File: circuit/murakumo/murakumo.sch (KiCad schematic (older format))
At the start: 105 parts, among them J1 Conn_01x03, J10 SWITCHandMOTORSIGNAL, J11 ENX_10_EASY_2, J2 Conn_01x03, J3 SWD, J4 FrontSensor, J5 I2C3, J6 LED, J7 ENX_10_EASY_1, J8 USART1, J9 Power, Q1 TEMT7100X01, Q10 2N7002T, Q11 TEMT7100X01, Q12 TEMT7100X01, Q13 TEMT7100X01, Q2 TEMT7100X01, Q3 TEMT7100X01, Q4 TEMT7100X01, Q5 TEMT7100X01, Q6 TEMT7100X01, Q7 TEMT7100X01, Q8 TEMT7100X01, Q9 TEMT7100X01, SW1 RST, U1 ASTMLPA-16MHz-LJ-E-T, U2 STM32F405RGTx, U3 ICM-20648

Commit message: hoge
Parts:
- removed U?: ASTMLPA-16MHz-LJ-E-T, symbol OSC:ASTMLPA-16MHz-LJ-E-T
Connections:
- net DRV1_EN: now also U2.54 (PD2); no longer U2.58 (PB6)
- net DRV1_PN: now also U2.58 (PB6); no longer U2.59 (PB7)
- net DRV1_nFAULT: now also U2.6 (PH1)
- net DRV1_nSLEEP: now also U2.2 (PC13)
- net DRV2_EN: no longer U2.61 (PB8)
- net DRV2_PN: now also U2.59 (PB7); no longer U2.62 (PB9)
- net DRV2_nFAULT: now also U2.3 (PC14)
- net DRV2_nSLEEP: now also U2.4 (PC15)
- net I2C3_SCL: no longer U2.41 (PA8)
- net I2C3_SDA: no longer U2.40 (PC9)
- net Rotary1: now also U2.45 (PA12); no longer U2.51 (PC10)
- net Rotary2: now also U2.44 (PA11); no longer U2.52 (PC11)
- net Rotary4: now also U2.43 (PA10); no longer U2.53 (PC12)
- net Rotary8: now also U2.34 (PB13); no longer U2.54 (PD2)
- net SW1: no longer U2.50 (PA15)
- net SW2: no longer U2.34 (PB13)
- net SW3: no longer U2.33 (PB12)
- net USART1_RX: no longer U2.43 (PA10)
- net USART1_TX: no longer U2.42 (PA9)
- net at R30.2: now also U2.50 (PA15); no longer U2.56 (PB4)
- net B renamed LED_B
- net LED_B: now also U2.53 (PC12); no longer U2.4 (PC15)
- net ENX1_A renamed Encorder1_A
- net Encorder1_A: now also U2.42 (PA9); no longer U2.44 (PA11)
- net ENX1_B renamed Encorder1_B
- net Encorder1_B: now also U2.41 (PA8); no longer U2.45 (PA12)
- net ENX2_A renamed Encorder2_A
- net Encorder2_A: now also U2.57 (PB5); no longer U2.37 (PC6)
- net ENX2_B renamed Encorder2_B
- net Encorder2_B: now also U2.56 (PB4); no longer U2.38 (PC7)
- net G renamed LED_G
- net LED_G: now also U2.52 (PC11); no longer U2.3 (PC14)
- net LED1 renamed LED1_White
- net LED1_White: no longer U2.57 (PB5)
- net LED2 renamed LED_Red
- net R renamed LED_R
- net LED_R: now also U2.51 (PC10); no longer U2.2 (PC13)
- new net ERV2_EN: U2.33 (PB12)
- new net I2C_SCL: U2.61 (PB8)
- new net I2C_SDA: U2.62 (PB9)
- new net LED_White1: U2.40 (PC9)
- new net USART_RX: U2.38 (PC7)
- new net USART_TX: U2.37 (PC6)
- no-connect marks 18 -> 17
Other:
- note added: "SensorBar"
- moved on the sheet: BZ1, C10, C11, C12, C13, C14, C17, C18, C19, D10, D11, D12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

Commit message: 次はフットプリントの関連付け
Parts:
- removed BZ1: TE044003-4, symbol Device:Buzzer
- removed C1, C12, C16, C17, C18, C2, C21, C22, C3, C4, C6, C7, C9: 0.1u, symbol Device:C
- removed C10, C11: 2.2u, symbol Device:C
- removed C13, C14, C15, C19, C20: C, symbol Device:C
- removed C5: 4.7u, symbol Device:C
- removed C8: 1u, symbol Device:C
- removed D1, D13, D14, D15, D2, D3, D4, D5, D6, D7, D8, D9: SIR19-21C/TR8, Diode_SMD:D_0603_1608Metric, symbol Device:LED
- removed D10, D11: LED, symbol Device:LED
- removed D12: RB751S40-AU_R1_000A1, symbol Device:D
- removed FB1, FB2, FB3: 470u, symbol Device:Ferrite_Bead
- removed J1, J2: Conn_01x03, symbol Connector_Generic:Conn_01x03
- removed J10: SWITCHandMOTORSIGNAL, symbol Connector_Generic:Conn_01x15
- removed J11: ENX_10_EASY_2, symbol Connector_Generic:Conn_02x05_Odd_Even
- removed J3: SWD, symbol Connector_Generic:Conn_01x06
- removed J4: FrontSensor, symbol Connector_Generic:Conn_01x06
- removed J5: I2C3, symbol Connector_Generic:Conn_01x04
- removed J6: LED, symbol Connector_Generic:Conn_01x05
- removed J7: ENX_10_EASY_1, symbol Connector_Generic:Conn_02x05_Odd_Even
- removed J8: USART1, symbol Connector_Generic:Conn_01x04
- removed J9: Power, symbol Connector_Generic:Conn_01x03
- removed Q1, Q11, Q12, Q13, Q2, Q3, Q4, Q5, Q6, Q7, Q8, Q9: TEMT7100X01, TEMT7100X01:TEMT7100X01, symbol Device:Q_Photo_NPN
- removed Q10: 2N7002T, Package_TO_SOT_SMD:SOT-23, symbol Transistor_FET:2N7002
- removed R1, R11, R13, R15, R17, R24, R26, R28, R3, R5, R7, R9: 100, Resistor_SMD:R_0603_1608Metric, symbol Device:R
- removed R10, R12, R14, R16, R18, R2, R21, R22, R23, R25, R27, R29, R31, R4, R6, R8, R?: 10k, symbol Device:R
- removed R19, R20: 470, symbol Device:R
- removed R30: 100, symbol Device:R
- removed R32: 36, symbol Device:R
- removed RN1: 10k, symbol Device:R_Pack03
- removed RN2: 10k, symbol Device:R_Pack04
- removed SW1: RST, symbol Switch:SW_MEC_5G
- removed U1: ASTMLPA-16MHz-LJ-E-T, symbol OSC:ASTMLPA-16MHz-LJ-E-T
- removed U2: STM32F405RGTx, Package_QFP:LQFP-64_10x10mm_P0.5mm, symbol MCU_ST_STM32F4:STM32F405RGTx
- removed U3: ICM-20648, symbol ICM-20648:ICM-20648
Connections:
- no-connect marks 17 -> 0
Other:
- note removed: "1.5mA"
- note removed: "20mA"
- note removed: "240mA\n"
- note removed: "2mA"
- note removed: "36mA"
- note removed: "6.2mA\n"
- note removed: "90mA"
- note removed: "Buzzer"
- note removed: "ENCORDER"
- note removed: "ForegroundSensor"
- note removed: "I2C"
- note removed: "InertialSensor"
- note removed: "Oscillator"
- note removed: "PowerSupply"
- note removed: "SWD"
- note removed: "SensorBar"
- note removed: "SideSensor"
- note removed: "USART"

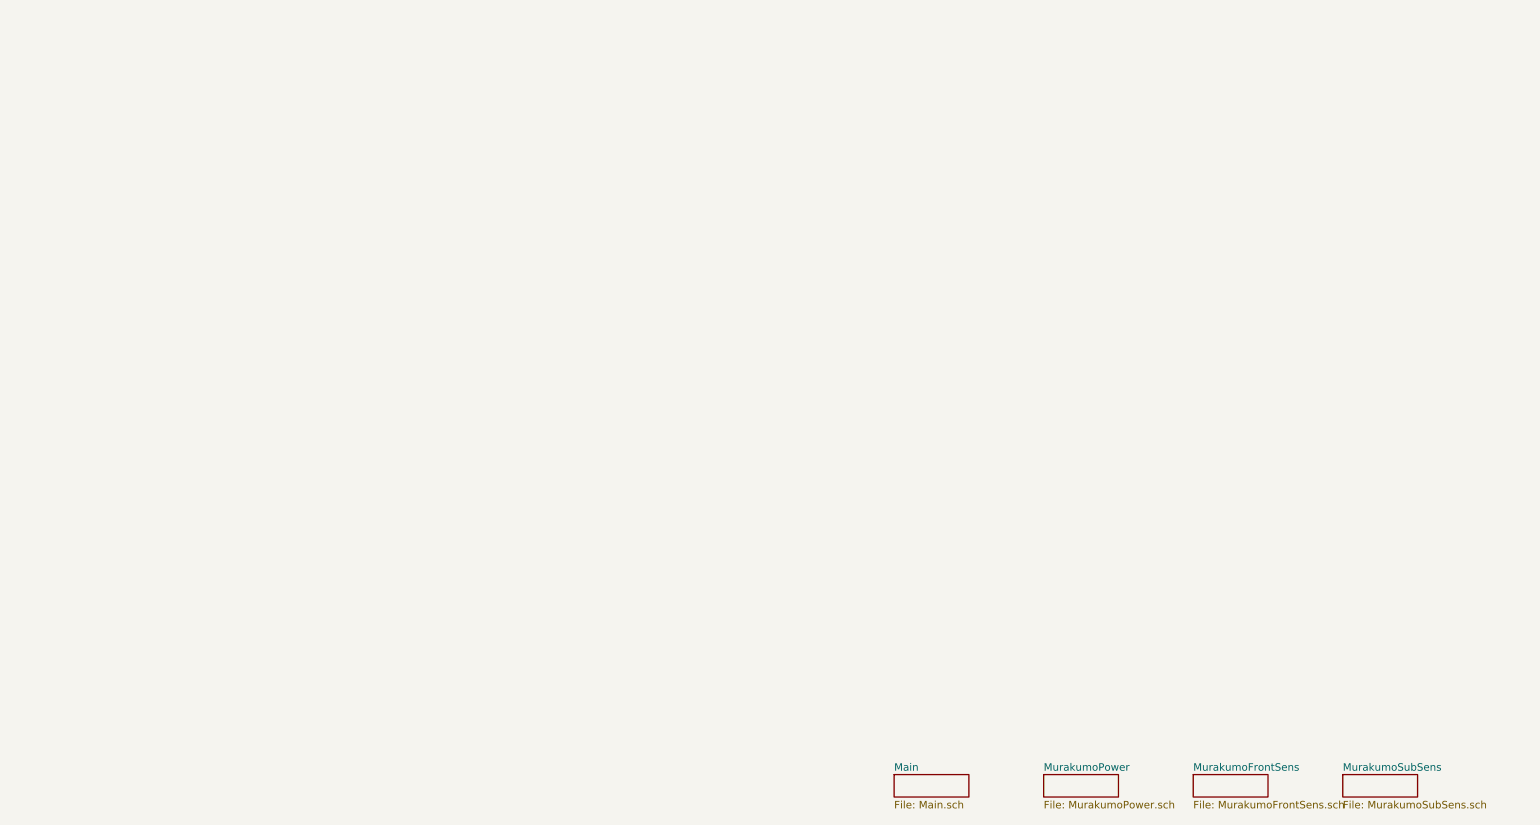
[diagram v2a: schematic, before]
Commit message: あとちょっとでフットプリントの関連付けが終わる
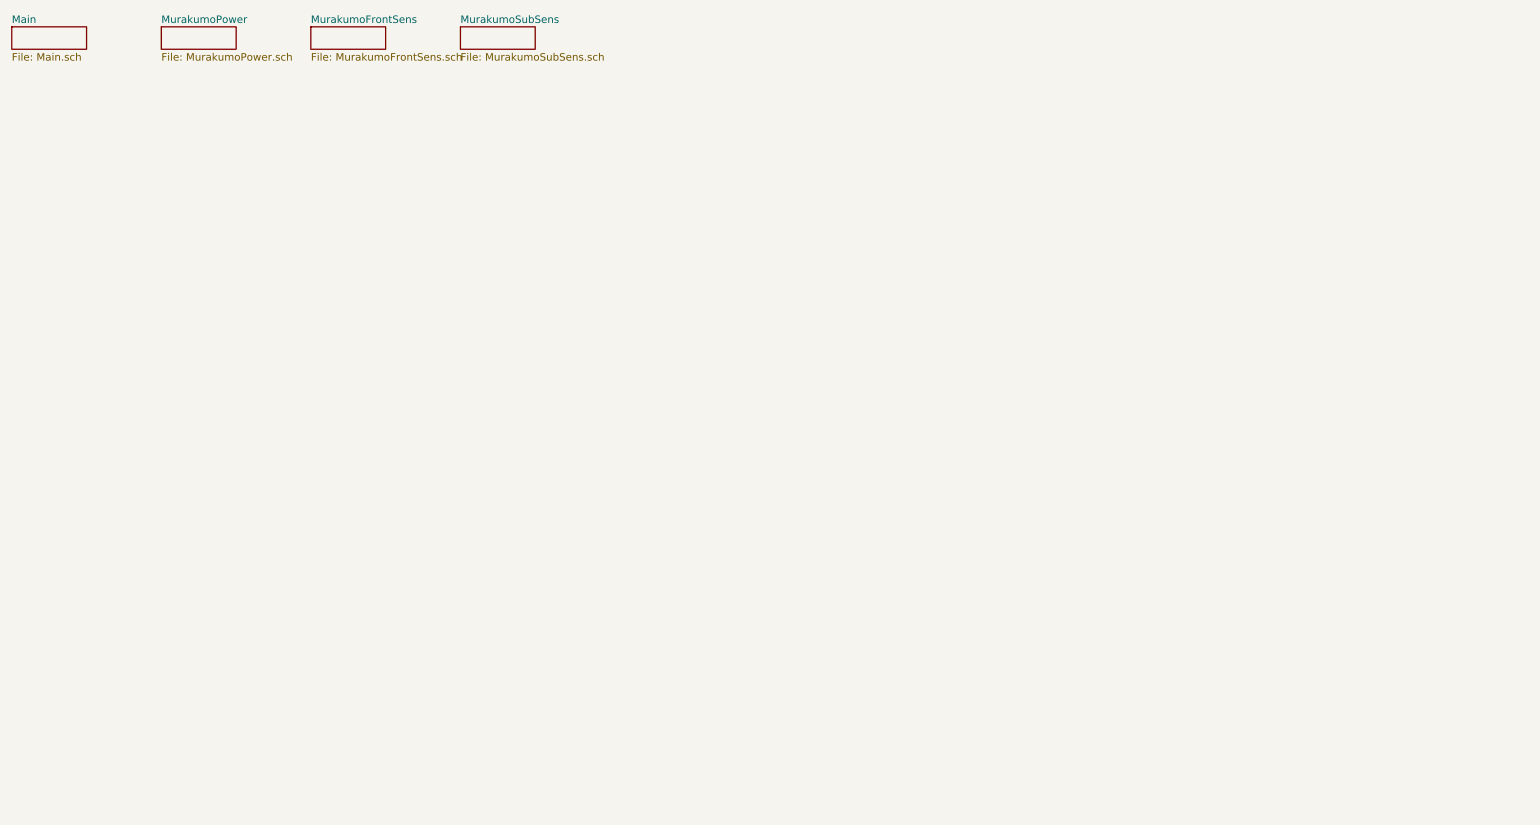
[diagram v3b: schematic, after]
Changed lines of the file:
@@
 EELAYER 30 0
 EELAYER END
-$Descr A2 23386 16535
+$Descr A4 11693 8268
 encoding utf-8
 Sheet 1 5
@@
 $EndDescr
 $Sheet
-S 11700 8950 500  150
+S 5800 3950 500  150
 U 61E3FF76
 F0 "MurakumoFrontSens" 50
@@
 $EndSheet
 $Sheet
-S 10700 8950 500  150
+S 4800 3950 500  150
 U 61EDC519
 F0 "MurakumoPower" 50
@@
 $EndSheet
 $Sheet
-S 12700 8950 500  150
+S 6800 3950 500  150
 U 61EC4080
 F0 "MurakumoSubSens" 50
@@
 $EndSheet
 $Sheet
-S 9700 8950 500  150
+S 3800 3950 500  150
 U 624FCD7A
 F0 "Main" 50
